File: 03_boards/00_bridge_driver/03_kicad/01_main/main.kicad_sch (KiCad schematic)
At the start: 2 parts, among them U5 STM32G431K8Tx, U6 MAX3485

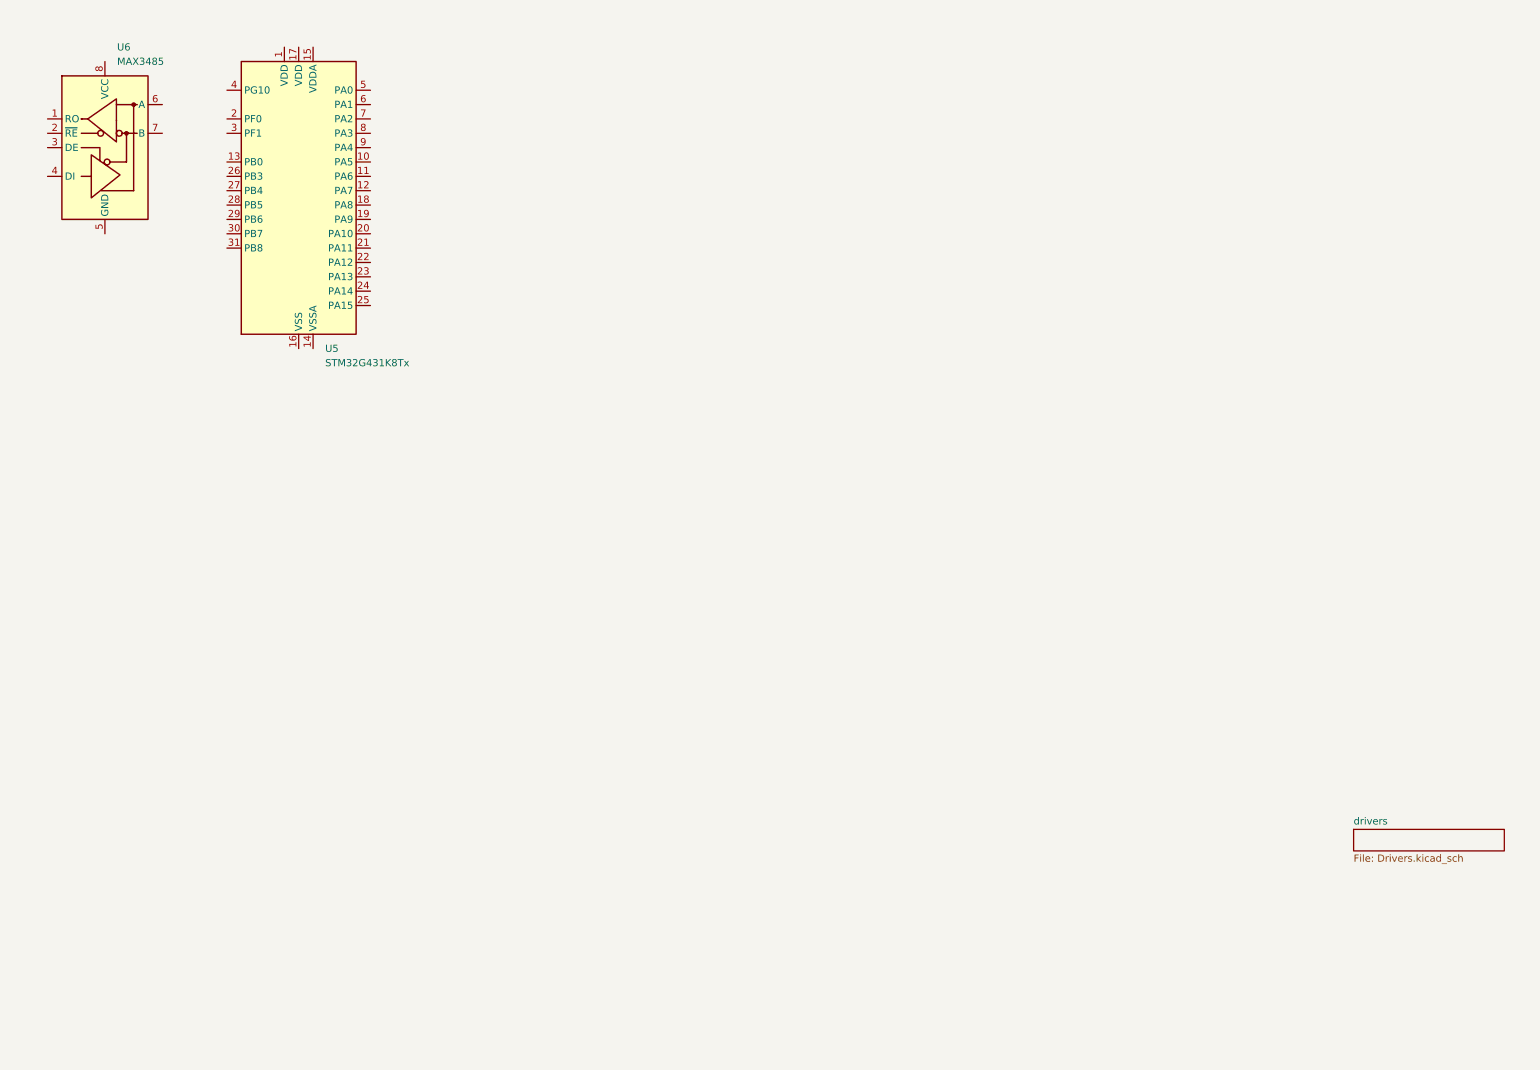
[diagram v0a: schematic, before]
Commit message: Week 0x8 | Simulation & Objectives (#34)
* Reordered motor folder and rewrote / cleaned up readmes within motors, boards and simulations

* Updated readme logo size

* Made logo 100% width

* Update scaled logo and removed finite element from readme

* Removed objectives

* Removed FEM from readme

* Removed Methodology

* Added a line break before prototype alpha image. Also removed figure naming from the document

* Trying a new formatting technique

* Moved boards link below image

* Removed `REV 2` from image description as its not needed

* Removing overview to see if its good or not

* Trying a new formatting style

* Removed the top line section

* Removed prototype from naming schema

* Changed top block

* Updated shields and updated description

* Removed some pose & added alpha and beta symbols because their cool

* Added a line break below documentation

* Added objectives to readme

* Removed the indexing from two notes

* Renamed `motor notes` with `alpha notes`

* Indexed the conceptual and removed : from note

* Updated parameter files and added short note about analytical model

* Cleaned up analytical model

* Updated analytical simulation

* Updated readmes for analytical model

* Updated the electrical equations

* Updated formatting for motors & boards

* Updated readmes and added sections to openLSM main readme

* I like it as a code block more

* Objectives should be in overview

* Moved aspirations note below objectives

* Made it more broad to contents than designs and contributions

* Updated subsection heading?

* Removed the "accurate dynamics" note its bad filler

* Removed TBD from readme

* Reformatting the tags section in documentation

* Updated analytical model

* Final iteration of analytical model before documentation

* Removing the global warning should be upto the individual readmes to say so

* Renamed metric.ut to derived.ut

* Added flow diagram for analytical model

* Updated the readmes to reflect uncertainty in the actual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
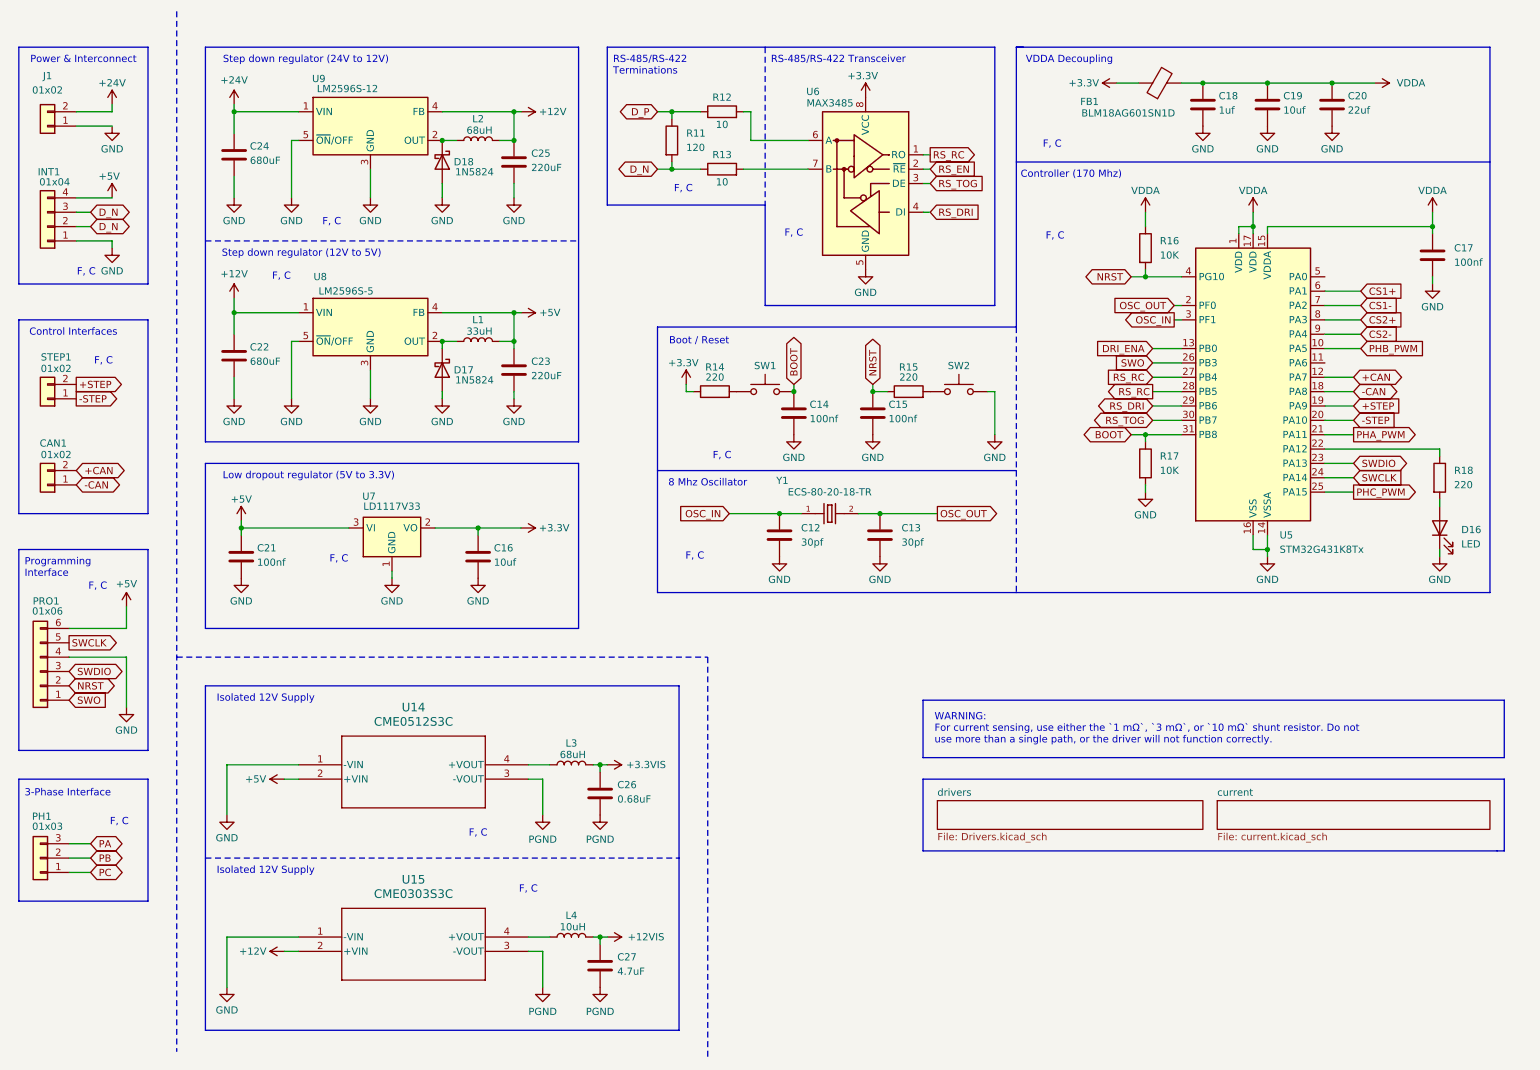
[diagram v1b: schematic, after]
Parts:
- added C12, C13: 30pf, symbol Device:C
- added C14, C15, C17, C21: 100nf, symbol Device:C
- added C16, C19: 10uf, symbol Device:C
- added C18: 1uf, symbol Device:C
- added C20: 22uf, symbol Device:C
- added C22, C24: 680uF, symbol Device:C
- added C23, C25: 220uF, symbol Device:C
- added C26: 0.68uF, symbol Device:C
- added C27: 4.7uF, symbol Device:C
- added CAN1, J1, STEP1: 01x02, symbol Connector_Generic:Conn_01x02
- added D16: LED, symbol Device:LED
- added D17, D18: 1N5824, Diode_THT:D_DO-201AD_P15.24mm_Horizontal, symbol Diode:1N5822
- added FB1: BLM18AG601SN1D, symbol Device:FerriteBead
- added INT1: 01x04, symbol Connector_Generic:Conn_01x04
- added L1: 33uH, symbol Device:L
- added L2, L3: 68uH, symbol Device:L
- added L4: 10uH, symbol Device:L
- added PH1: 01x03, symbol Connector_Generic:Conn_01x03
- added PRO1: 01x06, symbol Connector_Generic:Conn_01x06
- added R11: 120, symbol Device:R
- added R12, R13: 10, symbol Device:R
- added R14, R15, R18: 220, symbol Device:R
- added R16, R17: 10K, symbol Device:R
- added SW1, SW2: SW_Push, symbol Switch:SW_Push
- added U14: CME0512S3C, CME_SC_MUR, symbol 2026-08-29_14-59-18:CME0512S3C
- added U15: CME0303S3C, CME_SC_MUR, symbol 2026-08-29_14-59-18:CME0512S3C
- added U7: LD1117V33, Package_TO_SOT_THT:TO-220-3_Vertical, symbol Regulator_Linear:LD1117V33
- added U8: LM2596S-5, Package_TO_SOT_SMD:TO-263-5_TabPin3, symbol Regulator_Switching:LM2596S-5
- added U9: LM2596S-12, Package_TO_SOT_SMD:TO-263-5_TabPin3, symbol Regulator_Switching:LM2596S-12
- added Y1: ECS-80-20-18-TR, ECS-80-20-18-TR:XTAL_ECS-80-20-18-TR, symbol ECS-80-20-18-TR:ECS-80-20-18-TR
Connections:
- net RS_RC: now reaches U6.1 (RO)
- net RS_RC: now also U5.27 (PB4), U5.28 (PB5)
- net RS_EN: now reaches U6.2 (~{RE})
- net RS_TOG: now reaches U6.3 (DE)
- net RS_TOG: now also U5.30 (PB7)
- net RS_DRI: now reaches U6.4 (DI)
- net RS_DRI: now also U5.29 (PB6)
- net GND: now reaches U6.5 (GND)
- net GND: now also U5.14 (VSSA), U5.16 (VSS), U5.32 (VSS), C12.2, C13.2, C14.2, C15.2, C16.2, C17.2, C18.2, C19.2, C20.2, C21.2, C22.2, C23.2, C24.2, C25.2, D16.1 (K), D17.2 (A), D18.2 (A), INT1.1 (Pin_1), J1.1 (Pin_1), PRO1.4 (Pin_4), R17.2, SW2.2, U14.1 (-VIN), U15.1 (-VIN), U7.1 (GND), U8.3 (GND), U8.5 (~{ON}/OFF), U9.3 (GND), U9.5 (~{ON}/OFF)
- net at U6.6 (A): now also R12.2
- net at U6.7 (B): now also R13.2
- net +3.3V: now reaches U6.8 (VCC)
- net +3.3V: now also C16.1, FB1.1, R14.1, U7.2 (VO)
- net VDDA: now reaches U5.1 (VDD)
- net VDDA: now also U5.15 (VDDA), U5.17 (VDD), C17.1, C18.1, C19.1, C20.1, FB1.2, R16.1
- net PHB_PWM: now reaches U5.10 (PA5)
- net +CAN: now reaches U5.12 (PA7)
- net +CAN: now also CAN1.2 (Pin_2)
- net DRI_ENA: now reaches U5.13 (PB0)
- net -CAN: now reaches U5.18 (PA8)
- net -CAN: now also CAN1.1 (Pin_1)
- net +STEP: now reaches U5.19 (PA9)
- net +STEP: now also STEP1.2 (Pin_2)
- net OSC_OUT: now reaches U5.2 (PF0)
- net OSC_OUT: now also C13.1, Y1.2, Y1.3
- net -STEP: now reaches U5.20 (PA10)
- net -STEP: now also STEP1.1 (Pin_1)
- net PHA_PWM: now reaches U5.21 (PA11)
- net at U5.22 (PA12): now also R18.1
- net SWDIO: now reaches U5.23 (PA13)
- net SWDIO: now also PRO1.3 (Pin_3)
- net SWCLK: now reaches U5.24 (PA14)
- net SWCLK: now also PRO1.5 (Pin_5)
- net PHC_PWM: now reaches U5.25 (PA15)
- net SWO: now reaches U5.26 (PB3)
- net SWO: now also PRO1.1 (Pin_1)
- net OSC_IN: now reaches U5.3 (PF1)
- net OSC_IN: now also C12.1, Y1.1, Y1.4
- net BOOT: now reaches U5.31 (PB8)
- net BOOT: now also C14.1, R17.1, SW1.2
- net NRST: now reaches U5.4 (PG10)
- net NRST: now also C15.1, PRO1.2 (Pin_2), R15.1, R16.2
- net CS1+: now reaches U5.6 (PA1)
- net CS1-: now reaches U5.7 (PA2)
- net CS2+: now reaches U5.8 (PA3)
- net CS2-: now reaches U5.9 (PA4)
- new net: L4.1, U15.4 (+VOUT)
- new net: D17.1 (K), L1.1, U8.2 (OUT)
- new net: R14.2, SW1.1
- new net: D16.2 (A), R18.2
- new net: R15.2, SW2.1
- new net: D18.1 (K), L2.1, U9.2 (OUT)
- new net: L3.1, U14.4 (+VOUT)
- new net +12V: C22.1, C25.1, L2.2, U15.2 (+VIN), U8.1 (VIN), U9.4 (FB)
- new net +12VIS: C27.1, L4.2
- new net +24V: C24.1, J1.2 (Pin_2), U9.1 (VIN)
- new net +3.3VIS: C26.1, L3.2
- new net +5V: C21.1, C23.1, INT1.4 (Pin_4), L1.2, PRO1.6 (Pin_6), U14.2 (+VIN), U7.3 (VI), U8.4 (FB)
- new net D_N: INT1.2 (Pin_2), INT1.3 (Pin_3), R11.2, R13.1
- new net D_P: R11.1, R12.1
- new net PA: PH1.3 (Pin_3)
- new net PB: PH1.2 (Pin_2)
- new net PC: PH1.1 (Pin_1)
- new net PGND: C26.2, C27.2, U14.3 (-VOUT), U15.3 (-VOUT)
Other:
- added sheet current (current.kicad_sch)
- note added: "3-Phase Interface"
- note added: "8 Mhz Oscillator"
- note added: "Boot / Reset"
- note added: "Control Interfaces"
- note added: "Controller (170 Mhz)"
- note added: "F, C"
- note added: "Isolated 12V Supply"
- note added: "Low dropout regulator (5V to 3.3V)"
- note added: "Power & Interconnect"
- note added: "Programming Interface"
- note added: "RS-485/RS-422 Terminations"
- note added: "RS-485/RS-422 Transceiver"
- note added: "Step down regulator (12V to 5V)"
- note added: "Step down regulator (24V to 12V)"
- note added: "VDDA Decoupling"
- note added: "WARNING: For current sensing, use either the `1 mΩ`, `3 mΩ`, or `10 mΩ` shunt resistor. Do not use more than a single path, or the driver will not function correctly."
- moved on the sheet: U5, U6
